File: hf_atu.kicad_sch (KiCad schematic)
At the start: 107 parts, among them J10 TO SWR_IN, J11 TO FILT_OUT, J7 TO ANTENNA, J8 SWR_IN, J9 To CTRL:ATU, K13 G6E, K14 G6E, K15 G6E, K16 G6E, K17 G6E, K18 G6E, K19 G6E, K20 G6E, K21 G6E, K22 G6E, K23 G6E, K24 G6E, K25 G6E, K26 G6E, K27 G6E, K28 G6E, K29 G6E, T1 SWR, U10 ULN2803A, U6 MCP23017_SO, U7 ULN2803A, U8 ULN2803A

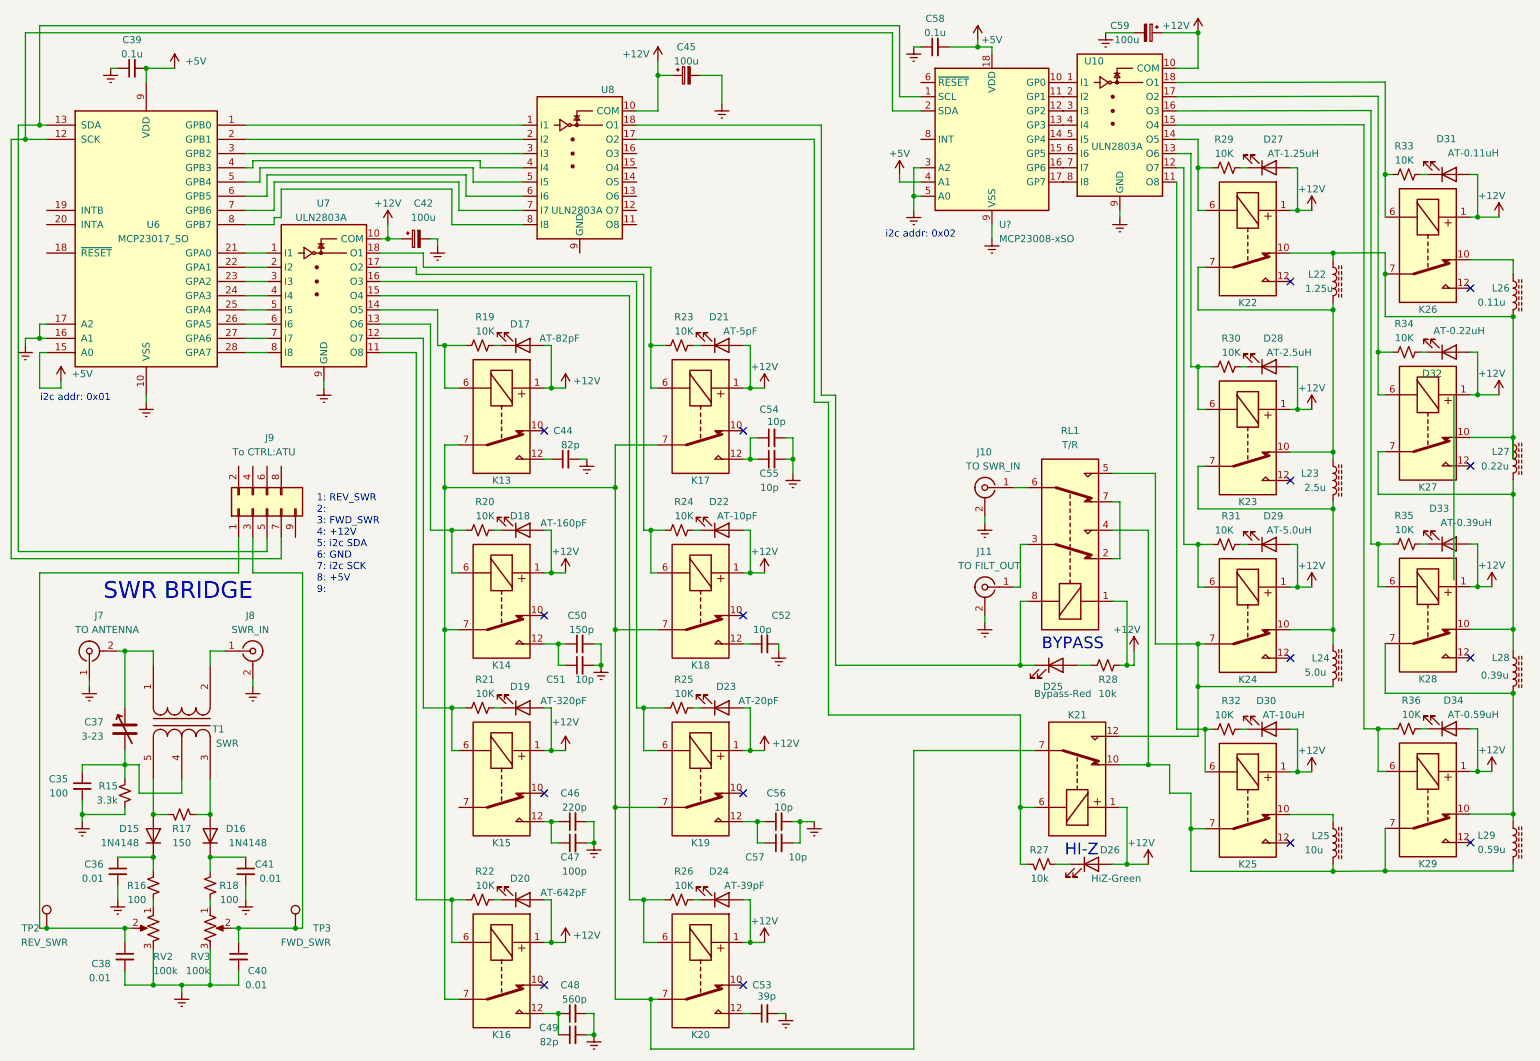
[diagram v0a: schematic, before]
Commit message: cleanup of schematic and some initial firmware works...
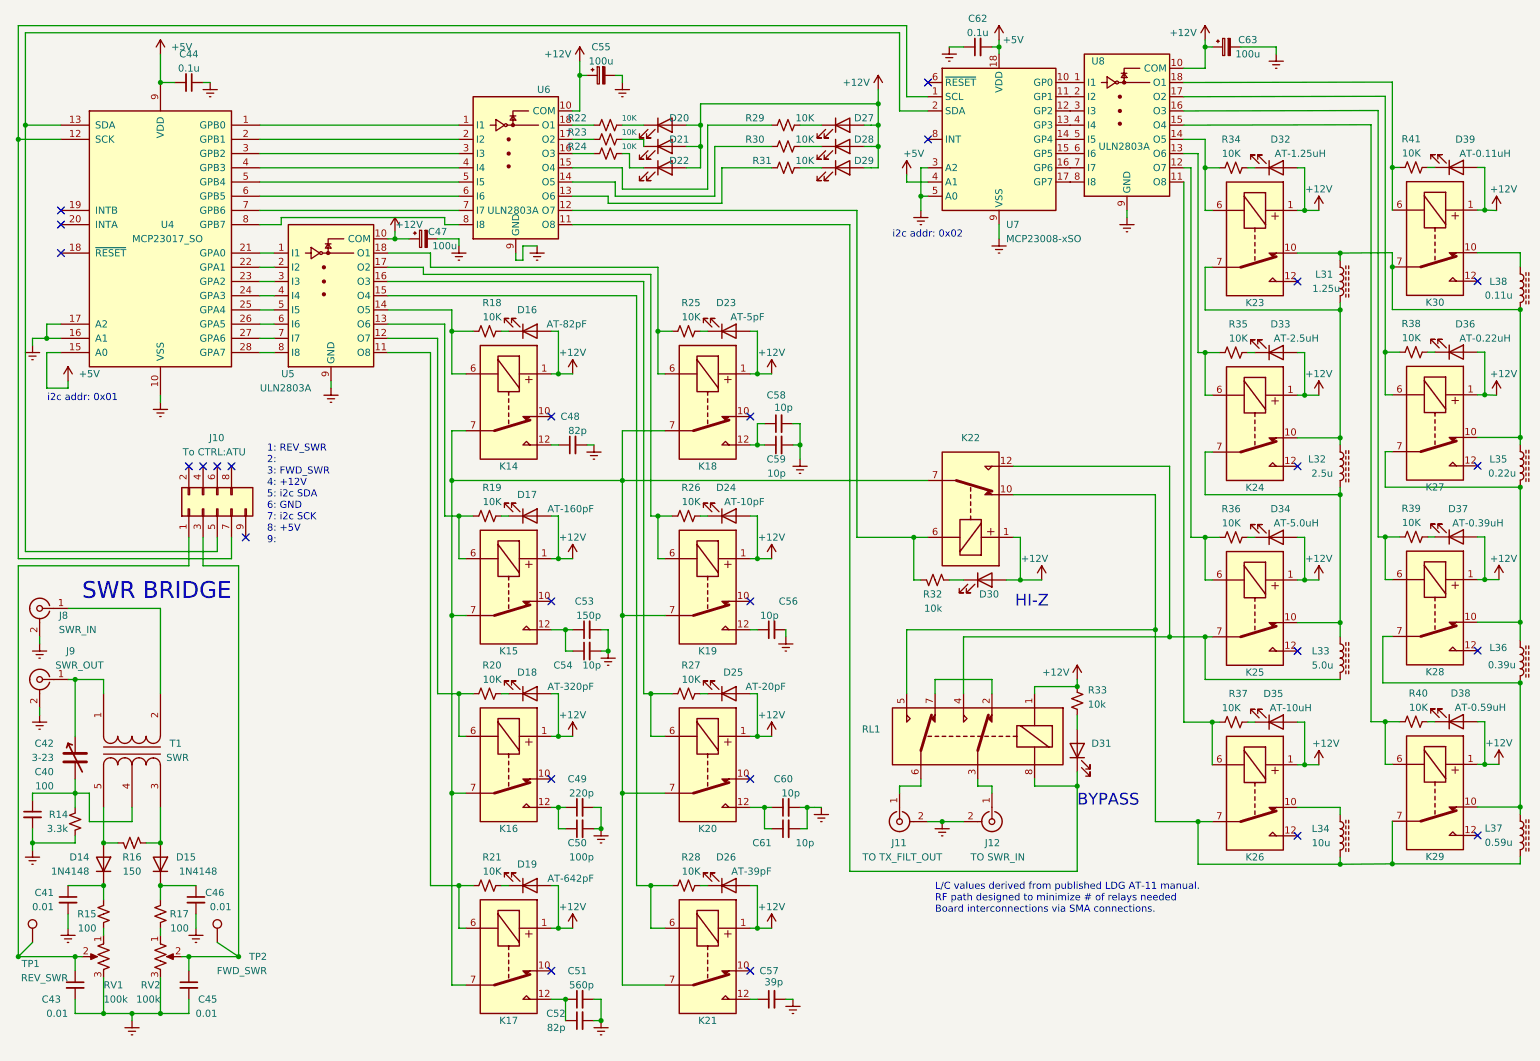
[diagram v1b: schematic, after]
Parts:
- removed D25: Bypass-Red, symbol Device:LED
- removed D26: HiZ-Green, symbol Device:LED
- removed J10: TO SWR_IN, symbol Connector:Conn_Coaxial
- removed K21: G6E, Relay_THT:Relay_SPDT_Omron_G6E, symbol Relay:G6E
- removed R27, R28: 10k, symbol Device:R_Small_US
- added D20, D21, D22, D27, D28, D29: LED, symbol Device:LED
- added D30: HiZ-Green, symbol Device:LED
- added D31: Bypass-Red, symbol Device:LED
- added J12: TO SWR_IN, symbol Connector:Conn_Coaxial
- added K22: G6E, Relay_THT:Relay_SPDT_Omron_G6E, symbol Relay:G6E
- added R22, R23, R24, R29, R30, R31: 10K, symbol Device:R_Small_US
- added R32, R33: 10k, symbol Device:R_Small_US
- J11: value TO FILT_OUT -> TO TX_FILT_OUT
- J9: renamed from J7; value TO ANTENNA -> SWR_OUT
- RL1: value T/R -> Bypass
- gave numbers to parts that had none: 1
- renumbered C35 to C40, C36 to C41, C37 to C42, C38 to C43, C39 to C44, C40 to C45, C41 to C46, C42 to C47, C44 to C48, C46 to C49, C47 to C50, C48 to C51, C49 to C52, C50 to C53, C51 to C54, C45 to C55, C52 to C56, C53 to C57, C54 to C58, C55 to C59, C56 to C60, C57 to C61, C58 to C62, C59 to C63, D15 to D14, D16 to D15, D17 to D16, D18 to D17, D19 to D18, D20 to D19, D21 to D23, D22 to D24, D23 to D25, D24 to D26, D27 to D32, D28 to D33, D29 to D34, D30 to D35, D32 to D36, D33 to D37, D34 to D38, D31 to D39, J9 to J10, K13 to K14, K14 to K15, K15 to K16, K16 to K17, K17 to K18, K18 to K19, K19 to K20, K20 to K21, K22 to K23, K23 to K24, K24 to K25, K25 to K26, K26 to K30, L22 to L31, L23 to L32, L24 to L33, L25 to L34, L27 to L35, L28 to L36, L29 to L37, L26 to L38, R15 to R14, R16 to R15, R17 to R16, R18 to R17, R19 to R18, R20 to R19, R21 to R20, R22 to R21, R23 to R25, R24 to R26, R25 to R27, R26 to R28, R29 to R34, R30 to R35, R31 to R36, R32 to R37, R34 to R38, R35 to R39, R36 to R40, R33 to R41, RV2 to RV1, RV3 to RV2, TP2 to TP1, TP3 to TP2, U6 to U4, U7 to U5, U8 to U6, U10 to U8
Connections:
- net +12V: now also D20.2 (A), D21.2 (A), D22.2 (A), D27.2 (A), D28.2 (A), D29.2 (A), D30.2 (A), K22.1, R33.1
- net Earth: now also J9.2 (Ext), U6.9 (GND), J12.2 (Ext); no longer J9.1 (In)
- net at K26.7, K29.7, L34.2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: now also RL1.5, K22.10; no longer RL1.4
- net at K25.7, L33.2: now also RL1.4, K22.12; no longer RL1.5
- net at U6.17 (O2): now also R23.1
- net at K14.7, K15.7, K17.7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: now also K16.7, K22.7
- net at RL1.3: now also J12.1 (In); no longer J11.1 (In)
- net at RL1.6: now also J11.1 (In)
- net at U6.18 (O1): now also R22.1; no longer RL1.8
- net at J10.5 (Pin_5), U4.13 (SDA): now also U7.2 (SDA); no longer U7.1 (SCL)
- net at J10.7 (Pin_7), U4.12 (SCK): now also U7.1 (SCL); no longer U7.2 (SDA)
- net at U6.11 (O8): now also RL1.8, D31.1 (K)
- net at U6.12 (O7): now also K22.6, R32.1
- net at U6.13 (O6): now also R31.1
- net at U6.14 (O5): now also R30.1
- net at U6.15 (O4): now also R29.1
- net at U6.16 (O3): now also R24.1
- net at C42.1, T1.1 (AA): now also J9.1 (In); no longer J9.2 (Ext)
- new net: D27.1 (K), R29.2
- new net: D31.2 (A), R33.2
- new net: D20.1 (K), R22.2
- new net: D28.1 (K), R30.2
- new net: D30.1 (K), R32.2
- new net: D29.1 (K), R31.2
- new net: D21.1 (K), R23.2
- new net: D22.1 (K), R24.2
- no-connect marks 16 -> 26
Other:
- note added: "L/C values derived from published LDG AT-11 manual. RF path designed to minimize # of relays needed Board interconnections via SMA connections."
- moved on the sheet: C40, C41, C42, C43, C44, C45, C46, C47, C48, C49, C50, C51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

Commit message: cleanup
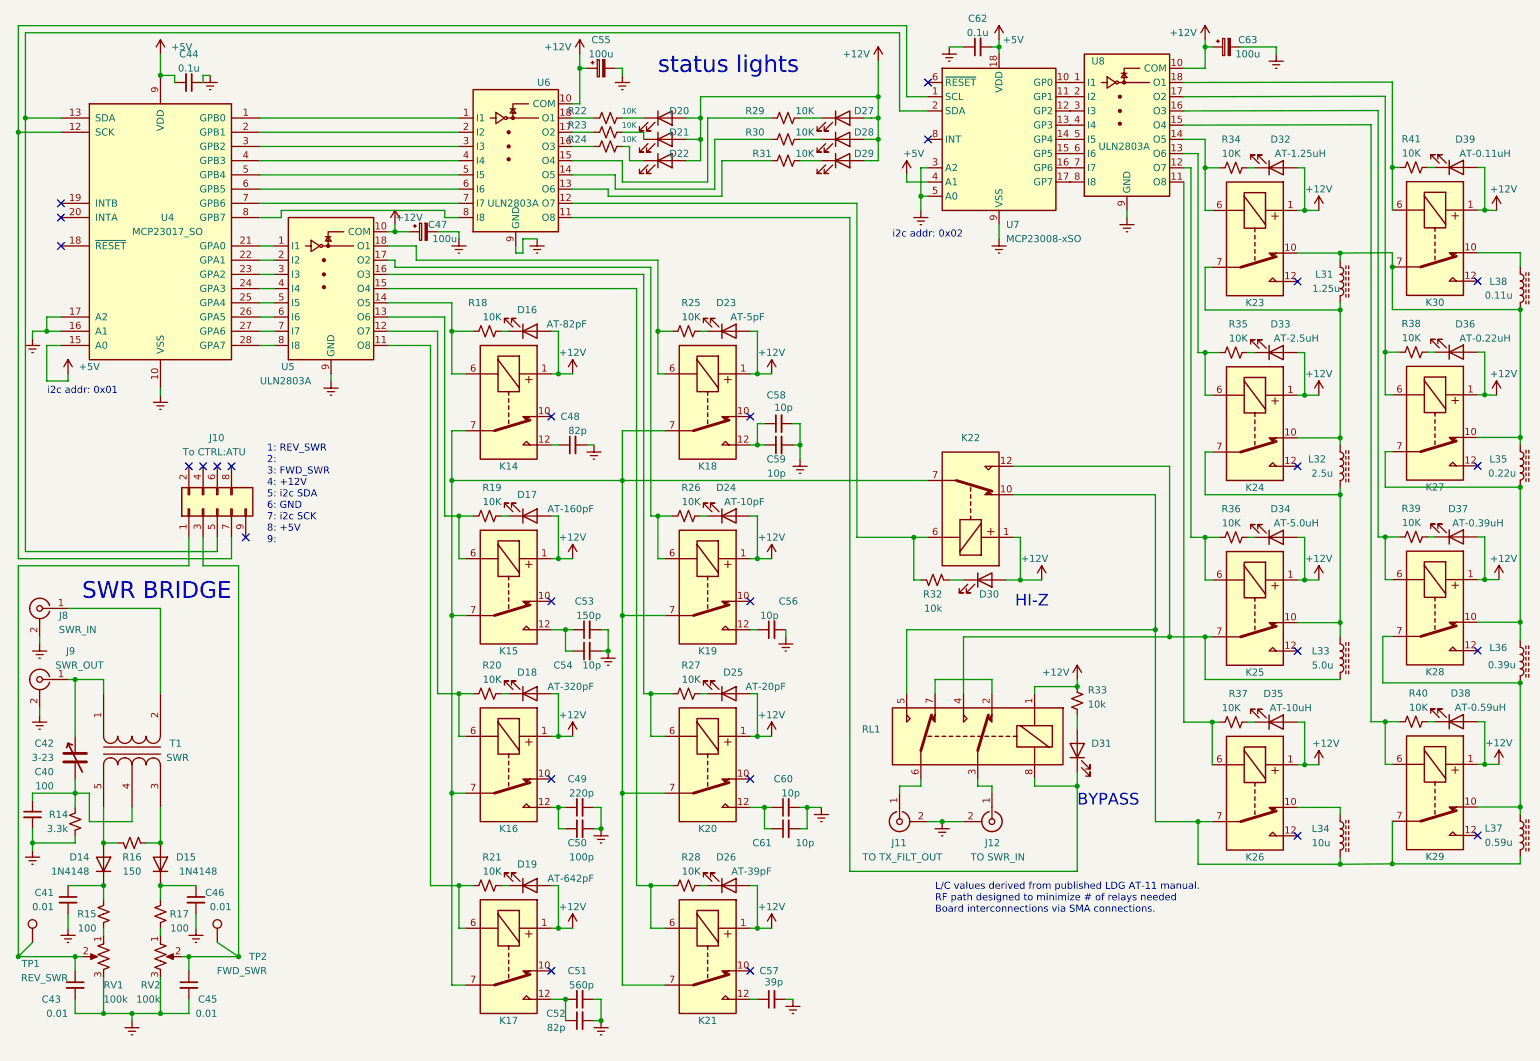
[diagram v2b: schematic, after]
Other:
- note added: "status lights"
- moved on the sheet: C47, C55, D20, D21, D22, D27, D28, D29, R22, R23, R24, R29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
